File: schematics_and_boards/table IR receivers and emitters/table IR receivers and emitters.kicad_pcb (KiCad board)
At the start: 2 copper layers, 80 x 28.1 mm, 29 parts, among them J1 Conn_Input, J2 Conn_Output, Q1 B17L1PT, Q2 B17L1PT, Q3 B17L1PT, Q4 B17L1PT, Q5 B17L1PT, Q6 B17L1PT, Q7 B17L1PT, Q8 B17L1PT, U1 74LV165PW-Q100J, U2 SN74HCS595PWR

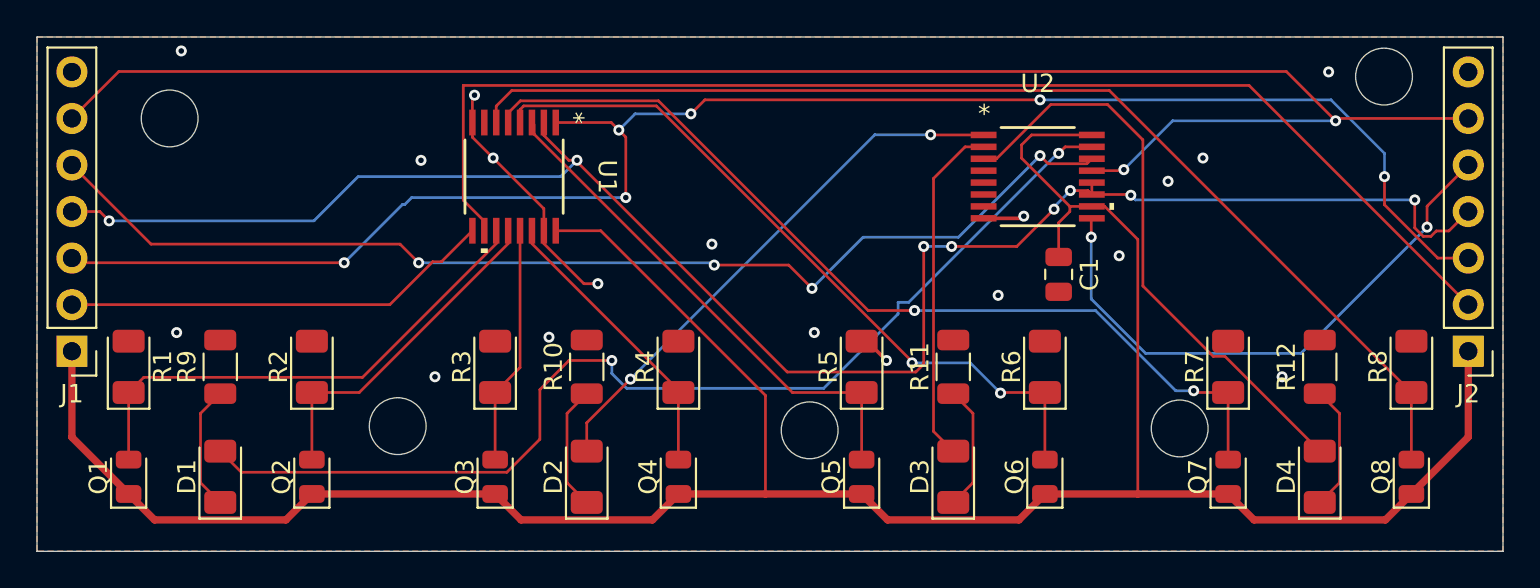
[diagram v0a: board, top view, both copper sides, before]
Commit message: initial designs for manufacture
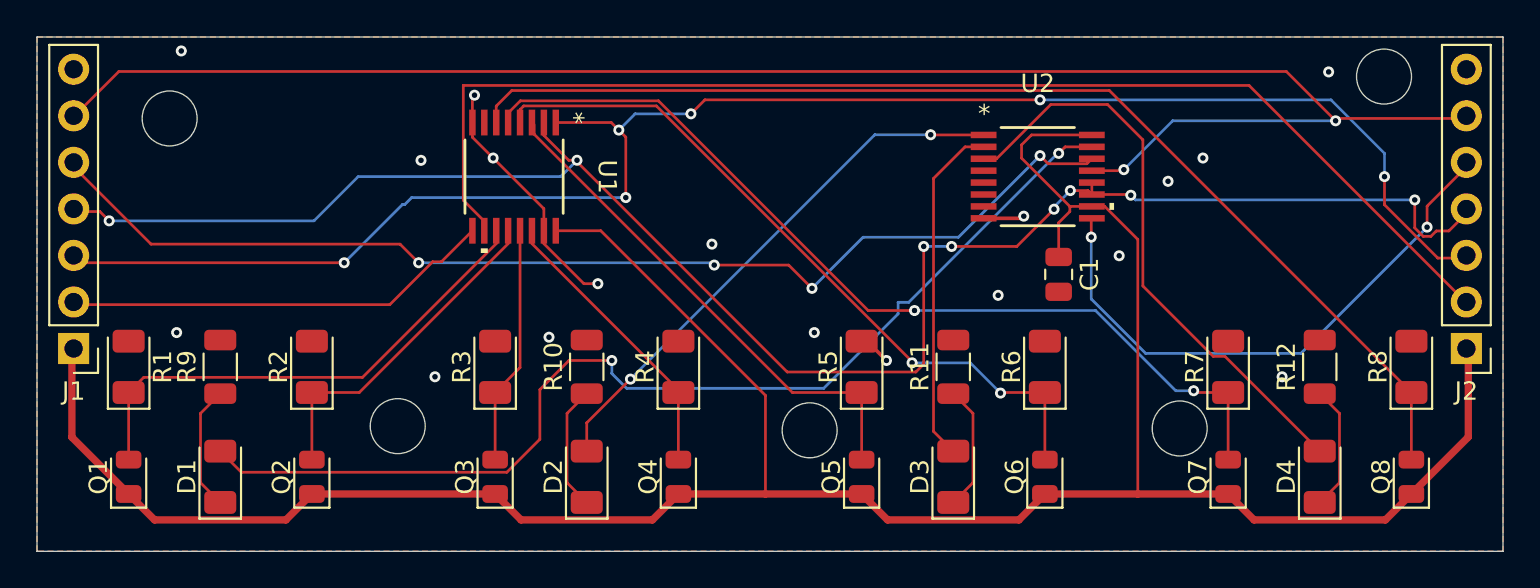
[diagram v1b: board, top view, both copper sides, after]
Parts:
- moved J2 0.18 mm to (178.3, 113.5)
- moved J1 0.17 mm to (102.3, 113.5)
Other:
- outline, holes or cut-outs redrawn
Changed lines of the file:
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@@
     )
     (pad_to_mask_clearance 0)
+    (grid_origin 100.33 96.52)
     (pcbplotparams
       (layerselection 0x00010fc_ffffffff)
@@
   (net 30 "unconnected-(U2-QH-Pad7)")
   (footprint "Connector_PinHeader_2.54mm:PinHeader_1x07_P2.54mm_Vertical" (layer "F.Cu")
-    (at 102.235 113.665 180)
+    (at 102.33 113.52 180)
     (descr "Through hole straight pin header, 1x07, 2.54mm pitch, single row")
     (tags "Through hole pin header THT 1x07 2.54mm single row")
@@
   )
   (footprint "Connector_PinHeader_2.54mm:PinHeader_1x07_P2.54mm_Vertical" (layer "F.Cu")
-    (at 178.435 113.665 180)
+    (at 178.33 113.52 180)
     (descr "Through hole straight pin header, 1x07, 2.54mm pitch, single row")
     (tags "Through hole pin header THT 1x07 2.54mm single row")
@@
     )
   )
-  (gr_circle (center 162.687 117.882) (end 164.237 117.882)
+  (gr_circle (center 162.687 117.882) (end 164.187 117.882)
     (stroke (width 0.0381) (type default)) (fill none) (layer "Edge.Cuts"))
-  (gr_circle (center 142.494 117.983) (end 144.044 117.983)
+  (gr_circle (center 142.494 117.983) (end 143.994 117.983)
     (stroke (width 0.0381) (type default)) (fill none) (layer "Edge.Cuts"))
-  (gr_circle (center 173.837 98.679) (end 175.387 98.679)
+  (gr_circle (center 173.837 98.679) (end 175.337 98.679)
     (stroke (width 0.0381) (type default)) (fill none) (layer "Edge.Cuts"))
-  (gr_circle (center 107.569 100.965) (end 109.119 100.965)
+  (gr_circle (center 107.569 100.965) (end 109.069 100.965)
     (stroke (width 0.0381) (type default)) (fill none) (layer "Edge.Cuts"))
   (gr_rect (start 100.33 96.52) (end 180.33 124.587)
     (stroke (width 0.0381) (type default)) (fill none) (layer "Edge.Cuts"))
-  (gr_circle (center 120.015 117.755) (end 121.565 117.755)
+  (gr_circle (center 120.015 117.755) (end 121.515 117.755)
     (stroke (width 0.0381) (type default)) (fill none) (layer "Edge.Cuts"))
   (gr_text "D&D Table IR Receiver/Emitter V1" (at 179.705 123.952) (layer "B.SilkS")
